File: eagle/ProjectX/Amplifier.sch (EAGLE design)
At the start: 5 parts, among them U1 TC4427COA

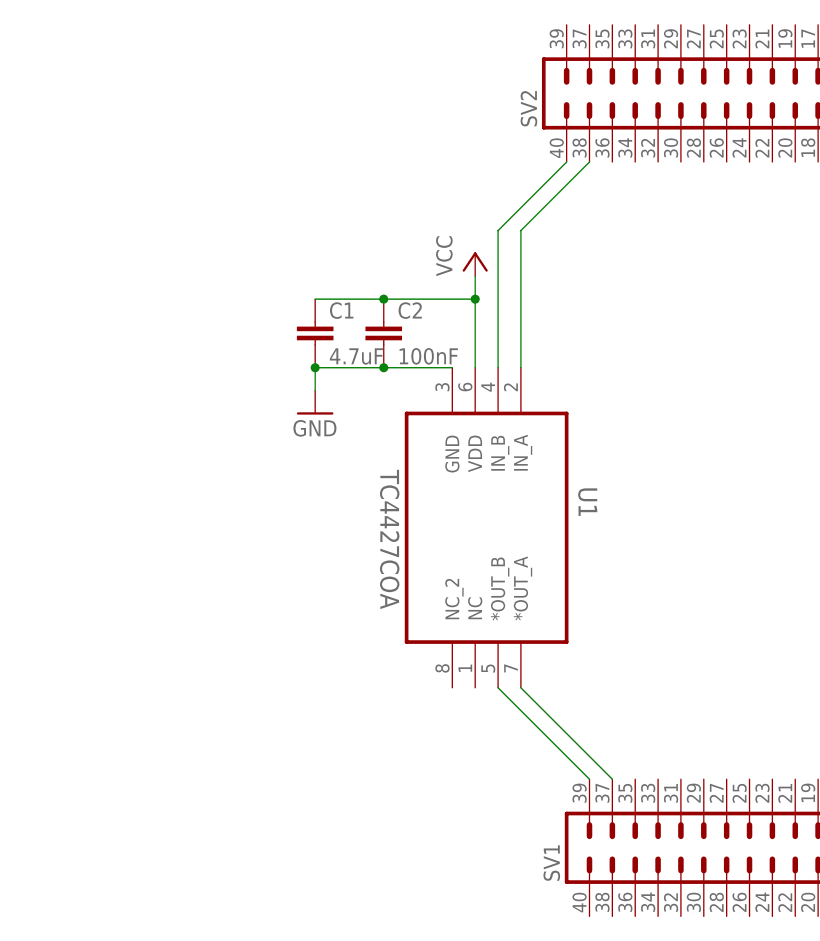
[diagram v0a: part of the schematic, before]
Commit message: Board update
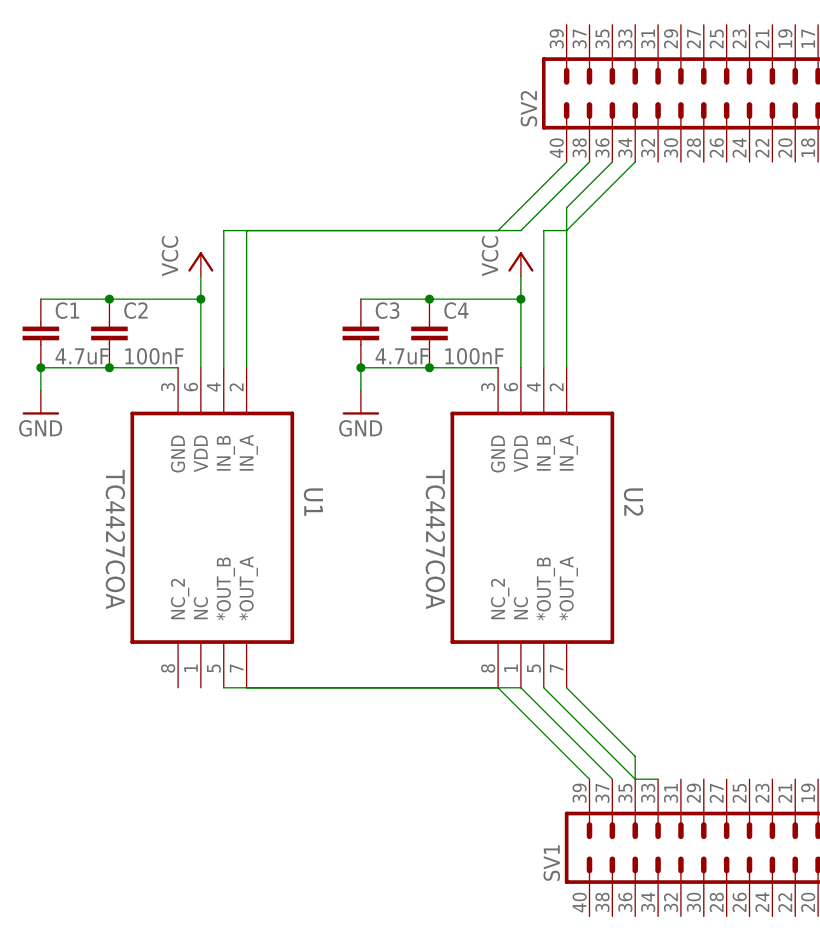
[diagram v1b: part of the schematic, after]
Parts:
- added C3: 4.7uF, rcl:C-EUC0805
- added C4: 100nF, rcl:C-EUC0805
- added U2: TC4427COA, Microchip_By_element14_Batch_1:TC4427COA
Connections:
- new net N$1: SV2.34, U2.IN_B
- new net N$6: SV2.36, U2.IN_A
- new net N$7: SV1.35, U2.*OUT_A
- new net N$8: SV1.33, U2.*OUT_B
- net GND: now also C3.2, C4.2, U2.GND
- net N$2: now also U1.*OUT_A; no longer U1.*OUT_B
- net N$3: now also U1.*OUT_B; no longer U1.*OUT_A
- net N$4: now also SV2.38; no longer SV2.40
- net N$5: now also SV2.40; no longer SV2.38
- net VCC: now also C3.1, C4.1, U2.VDD
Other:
- moved on the sheet: C1, C2, U1
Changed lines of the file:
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@@
 <part name="P+4" library="supply1" library_urn="urn:adsk.eagle:library:371" deviceset="VCC" device=""/>
 <part name="P+5" library="supply1" library_urn="urn:adsk.eagle:library:371" deviceset="VCC" device=""/>
+<part name="U2" library="Microchip_By_element14_Batch_1" deviceset="TC4427COA" device=""/>
+<part name="C3" library="rcl" library_urn="urn:adsk.eagle:library:334" deviceset="C-EU" device="C0805" package3d_urn="urn:adsk.eagle:package:23617/2" value="4.7uF"/>
+<part name="C4" library="rcl" library_urn="urn:adsk.eagle:library:334" deviceset="C-EU" device="C0805" package3d_urn="urn:adsk.eagle:package:23617/2" value="100nF"/>
+<part name="P+6" library="supply1" library_urn="urn:adsk.eagle:library:371" deviceset="VCC" device=""/>
+<part name="GND6" library="supply1" library_urn="urn:adsk.eagle:library:371" deviceset="GND" device=""/>
 </parts>
 <sheets>
@@
 </plain>
 <instances>
-<instance part="U1" gate="A" x="5.08" y="43.18" rot="R270"/>
-<instance part="C1" gate="G$1" x="-17.78" y="66.04"/>
-<instance part="C2" gate="G$1" x="-10.16" y="66.04"/>
+<instance part="U1" gate="A" x="-25.4" y="43.18" rot="R270"/>
+<instance part="C1" gate="G$1" x="-48.26" y="66.04"/>
+<instance part="C2" gate="G$1" x="-40.64" y="66.04"/>
 <instance part="SV1" gate="1" x="35.56" y="7.62" rot="R90"/>
 <instance part="SV2" gate="1" x="33.02" y="91.44" rot="R90"/>
@@
 <instance part="P+1" gate="VCC" x="58.42" y="22.86"/>
 <instance part="P+2" gate="VCC" x="58.42" y="-5.08" rot="R180"/>
-<instance part="P+3" gate="VCC" x="0" y="73.66"/>
-<instance part="GND3" gate="1" x="-17.78" y="55.88"/>
+<instance part="P+3" gate="VCC" x="-30.48" y="73.66"/>
+<instance part="GND3" gate="1" x="-48.26" y="55.88"/>
 <instance part="GND4" gate="1" x="58.42" y="104.14" rot="R180"/>
 <instance part="GND5" gate="1" x="58.42" y="76.2"/>
 <instance part="P+4" gate="VCC" x="55.88" y="78.74" rot="R180"/>
 <instance part="P+5" gate="VCC" x="55.88" y="111.76"/>
+<instance part="U2" gate="A" x="10.16" y="43.18" rot="R270"/>
+<instance part="C3" gate="G$1" x="-12.7" y="66.04"/>
+<instance part="C4" gate="G$1" x="-5.08" y="66.04"/>
+<instance part="P+6" gate="VCC" x="5.08" y="73.66"/>
+<instance part="GND6" gate="1" x="-12.7" y="55.88"/>
 </instances>
 <busses>
@@
 <pinref part="U1" gate="A" pin="VDD"/>
 <pinref part="P+3" gate="VCC" pin="VCC"/>
-<wire x1="0" y1="60.96" x2="0" y2="68.58" width="0.1524" layer="91"/>
+<wire x1="-30.48" y1="60.96" x2="-30.48" y2="68.58" width="0.1524" layer="91"/>
 <pinref part="C2" gate="G$1" pin="1"/>
-<wire x1="0" y1="68.58" x2="0" y2="71.12" width="0.1524" layer="91"/>
-<wire x1="0" y1="68.58" x2="-10.16" y2="68.58" width="0.1524" layer="91"/>
-<junction x="0" y="68.58"/>
+<wire x1="-30.48" y1="68.58" x2="-30.48" y2="71.12" width="0.1524" layer="91"/>
+<wire x1="-30.48" y1="68.58" x2="-40.64" y2="68.58" width="0.1524" layer="91"/>
+<junction x="-30.48" y="68.58"/>
 <pinref part="C1" gate="G$1" pin="1"/>
-<wire x1="-10.16" y1="68.58" x2="-17.78" y2="68.58" width="0.1524" layer="91"/>
-<junction x="-10.16" y="68.58"/>
+<wire x1="-40.64" y1="68.58" x2="-48.26" y2="68.58" width="0.1524" layer="91"/>
+<junction x="-40.64" y="68.58"/>
 </segment>
 <segment>
@@
 <pinref part="P+4" gate="VCC" pin="VCC"/>
 <wire x1="55.88" y1="83.82" x2="55.88" y2="81.28" width="0.1524" layer="91"/>
+</segment>
+<segment>
+<pinref part="U2" gate="A" pin="VDD"/>
+<pinref part="P+6" gate="VCC" pin="VCC"/>
+<wire x1="5.08" y1="60.96" x2="5.08" y2="68.58" width="0.1524" layer="91"/>
+<pinref part="C4" gate="G$1" pin="1"/>
+<wire x1="5.08" y1="68.58" x2="5.08" y2="71.12" width="0.1524" layer="91"/>
+<wire x1="5.08" y1="68.58" x2="-5.08" y2="68.58" width="0.1524" layer="91"/>
+<junction x="5.08" y="68.58"/>
+<pinref part="C3" gate="G$1" pin="1"/>
+<wire x1="-5.08" y1="68.58" x2="-12.7" y2="68.58" width="0.1524" layer="91"/>
+<junction x="-5.08" y="68.58"/>
 </segment>
 </net>
@@
 <pinref part="U1" gate="A" pin="GND"/>
 <pinref part="C2" gate="G$1" pin="2"/>
-<wire x1="-2.54" y1="60.96" x2="-10.16" y2="60.96" width="0.1524" layer="91"/>
+<wire x1="-33.02" y1="60.96" x2="-40.64" y2="60.96" width="0.1524" layer="91"/>
 <pinref part="C1" gate="G$1" pin="2"/>
-<wire x1="-10.16" y1="60.96" x2="-17.78" y2="60.96" width="0.1524" layer="91"/>
-<junction x="-10.16" y="60.96"/>
+<wire x1="-40.64" y1="60.96" x2="-48.26" y2="60.96" width="0.1524" layer="91"/>
+<junction x="-40.64" y="60.96"/>
 <pinref part="GND3" gate="1" pin="GND"/>
-<wire x1="-17.78" y1="58.42" x2="-17.78" y2="60.96" width="0.1524" layer="91"/>
-<junction x="-17.78" y="60.96"/>
+<wire x1="-48.26" y1="58.42" x2="-48.26" y2="60.96" width="0.1524" layer="91"/>
+<junction x="-48.26" y="60.96"/>
 </segment>
 <segment>
@@
 <wire x1="58.42" y1="83.82" x2="58.42" y2="78.74" width="0.1524" layer="91"/>
 </segment>
+<segment>
+<pinref part="U2" gate="A" pin="GND"/>
+<pinref part="C4" gate="G$1" pin="2"/>
+<wire x1="2.54" y1="60.96" x2="-5.08" y2="60.96" width="0.1524" layer="91"/>
+<pinref part="C3" gate="G$1" pin="2"/>
+<wire x1="-5.08" y1="60.96" x2="-12.7" y2="60.96" width="0.1524" layer="91"/>
+<junction x="-5.08" y="60.96"/>
+<pinref part="GND6" gate="1" pin="GND"/>
+<wire x1="-12.7" y1="58.42" x2="-12.7" y2="60.96" width="0.1524" layer="91"/>
+<junction x="-12.7" y="60.96"/>
+</segment>
 </net>
 <net name="N$4" class="0">
 <segment>
-<pinref part="SV2" gate="1" pin="40"/>
-<wire x1="10.16" y1="83.82" x2="2.54" y2="76.2" width="0.1524" layer="91"/>
-<wire x1="2.54" y1="76.2" x2="2.54" y2="60.96" width="0.1524" layer="91"/>
+<wire x1="-27.94" y1="76.2" x2="-27.94" y2="60.96" width="0.1524" layer="91"/>
 <pinref part="U1" gate="A" pin="IN_B"/>
+<pinref part="SV2" gate="1" pin="38"/>
+<wire x1="-27.94" y1="76.2" x2="5.08" y2="76.2" width="0.1524" layer="91"/>
+<wire x1="5.08" y1="76.2" x2="12.7" y2="83.82" width="0.1524" layer="91"/>
 </segment>
 </net>
 <net name="N$5" class="0">
 <segment>
-<pinref part="SV2" gate="1" pin="38"/>
-<wire x1="12.7" y1="83.82" x2="5.08" y2="76.2" width="0.1524" layer="91"/>
-<wire x1="5.08" y1="76.2" x2="5.08" y2="60.96" width="0.1524" layer="91"/>
+<wire x1="-25.4" y1="76.2" x2="-25.4" y2="60.96" width="0.1524" layer="91"/>
 <pinref part="U1" gate="A" pin="IN_A"/>
+<pinref part="SV2" gate="1" pin="40"/>
+<wire x1="-25.4" y1="76.2" x2="2.54" y2="76.2" width="0.1524" layer="91"/>
+<wire x1="2.54" y1="76.2" x2="10.16" y2="83.82" width="0.1524" layer="91"/>
+</segment>
+</net>
+<net name="N$1" class="0">
+<segment>
+<wire x1="7.62" y1="76.2" x2="7.62" y2="60.96" width="0.1524" layer="91"/>
+<pinref part="U2" gate="A" pin="IN_B"/>
+<pinref part="SV2" gate="1" pin="34"/>
+<wire x1="7.62" y1="76.2" x2="10.16" y2="76.2" width="0.1524" layer="91"/>
+<wire x1="10.16" y1="76.2" x2="17.78" y2="83.82" width="0.1524" layer="91"/>
+</segment>
+</net>
+<net name="N$7" class="0">
+<segment>
+<pinref part="SV1" gate="1" pin="35"/>
+<pinref part="U2" gate="A" pin="*OUT_A"/>
+<wire x1="17.78" y1="15.24" x2="17.78" y2="17.78" width="0.1524" layer="91"/>
+<wire x1="17.78" y1="17.78" x2="10.16" y2="25.4" width="0.1524" layer="91"/>
+</segment>
+</net>
+<net name="N$8" class="0">
+<segment>
+<pinref part="SV1" gate="1" pin="33"/>
+<pinref part="U2" gate="A" pin="*OUT_B"/>
+<wire x1="20.32" y1="15.24" x2="17.78" y2="15.24" width="0.1524" layer="91"/>
+<wire x1="17.78" y1="15.24" x2="7.62" y2="25.4" width="0.1524" layer="91"/>
+</segment>
+</net>
+<net name="N$6" class="0">
+<segment>
+<pinref part="U2" gate="A" pin="IN_A"/>
+<pinref part="SV2" gate="1" pin="36"/>
+<wire x1="10.16" y1="60.96" x2="10.16" y2="78.74" width="0.1524" layer="91"/>
+<wire x1="10.16" y1="78.74" x2="15.24" y2="83.82" width="0.1524" layer="91"/>
 </segment>
 </net>
 <net name="N$2" class="0">
 <segment>
-<pinref part="U1" gate="A" pin="*OUT_B"/>
+<pinref part="U1" gate="A" pin="*OUT_A"/>
 <pinref part="SV1" gate="1" pin="39"/>
+<wire x1="-25.4" y1="25.4" x2="2.54" y2="25.4" width="0.1524" layer="91"/>
 <wire x1="2.54" y1="25.4" x2="12.7" y2="15.24" width="0.1524" layer="91"/>
 </segment>
@@
 <net name="N$3" class="0">
 <segment>
-<pinref part="U1" gate="A" pin="*OUT_A"/>
+<pinref part="U1" gate="A" pin="*OUT_B"/>
 <pinref part="SV1" gate="1" pin="37"/>
+<wire x1="-27.94" y1="25.4" x2="5.08" y2="25.4" width="0.1524" layer="91"/>
 <wire x1="5.08" y1="25.4" x2="15.24" y2="15.24" width="0.1524" layer="91"/>
 </segment>

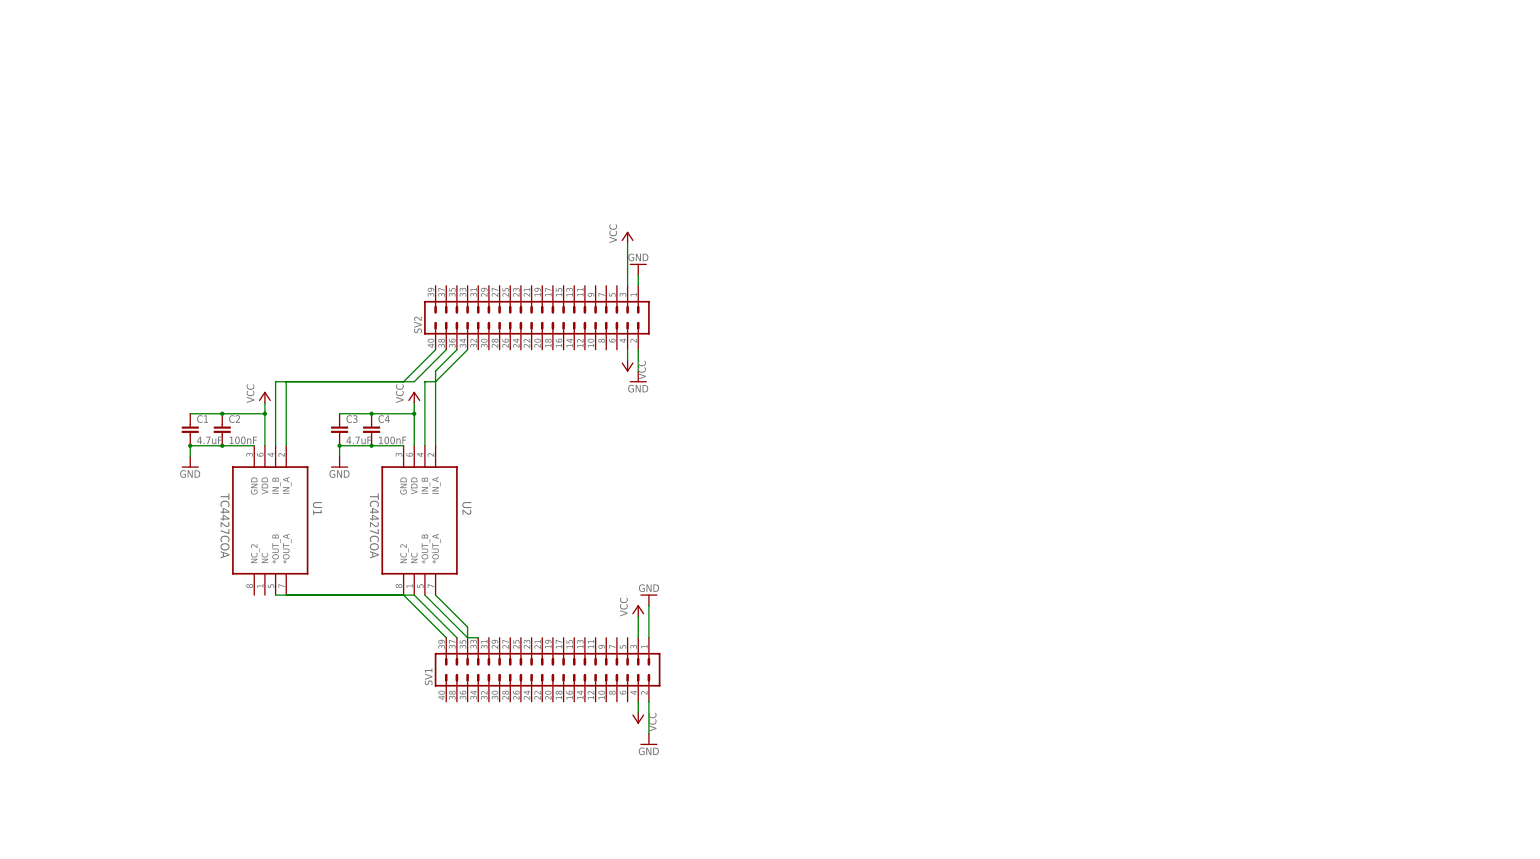
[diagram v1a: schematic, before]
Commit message: changes
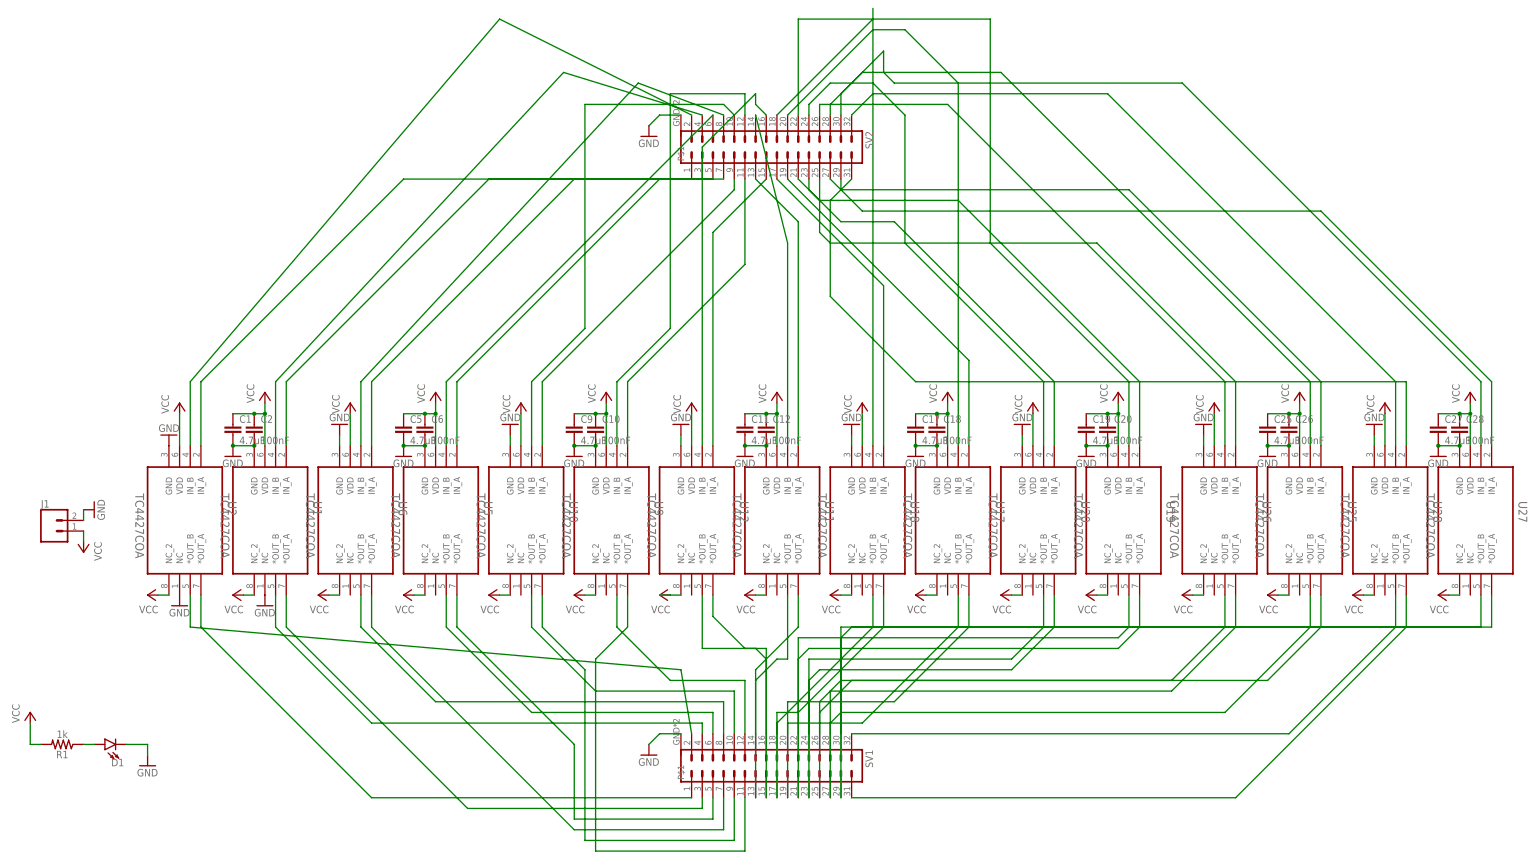
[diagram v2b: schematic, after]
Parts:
- removed C3: 4.7uF, rcl:C-EUC0805
- removed C4: 100nF, rcl:C-EUC0805
- added C10, C12, C18, C20, C26, C28, C6: 100nF, rcl:C-EUC0805
- added C11, C17, C19, C25, C27, C5, C9: 4.7uF, rcl:C-EUC0805
- added D1: (no value), SparkFun-LED:LED0603
- added J1: (no value), SparkFun-Connectors:CONN_02PTH3
- added R1: 1k, SparkFun-Resistors:0.22OHM-0805-1/4W-1%
- added U10, U11, U12, U17, U18, U19, U20, U25, U26, U27, U28, U5, U6, U9: TC4427COA, Microchip_By_element14_Batch_1:TC4427COA
- SV1, SV2: device con-lstb:MA20-2W -> Parts:MA20-2W
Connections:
- removed net VCC: C1.1, C2.1, C3.1, C4.1, SV1.3, SV1.4, SV2.3, SV2.4, U1.VDD, U2.VDD
- new net N$10: SV1.1, U2.*OUT_A
- new net N$100: SV1.25, U26.*OUT_A
- new net N$101: SV1.26, U26.*OUT_B
- new net N$102: SV2.25, U26.IN_A
- new net N$103: SV1.27, U25.*OUT_A
- new net N$104: SV1.28, U25.*OUT_B
- new net N$105: SV2.30, U27.IN_B
- new net N$106: SV2.29, U27.IN_A
- new net N$107: SV2.32, U28.IN_B
- new net N$108: SV1.31, U28.*OUT_A
- new net N$109: SV1.32, U28.*OUT_B
- new net N$11: SV1.3, U1.*OUT_A
- new net N$110: SV2.31, U28.IN_A
- new net N$111: SV1.29, U27.*OUT_A
- new net N$112: SV1.30, U27.*OUT_B
- new net N$12: SV1.7, U6.*OUT_A
- new net N$13: SV1.10, U10.*OUT_B
- new net N$14: SV1.9, U10.*OUT_A
- new net N$15: SV1.11, U9.*OUT_A
- new net N$16: SV1.23, U20.*OUT_A
- new net N$17: SV2.6, U5.IN_B
- new net N$18: SV2.5, U5.IN_A
- new net N$19: SV2.8, U6.IN_B
- new net N$20: D1.A, R1.1
- new net N$22: SV2.7, U6.IN_A
- new net N$23: SV1.5, U5.*OUT_A
- new net N$24: SV1.6, U5.*OUT_B
- new net N$26: SV1.15, U12.*OUT_A
- new net N$29: SV1.12, U9.*OUT_B
- new net N$33: SV2.12, U9.IN_B
- new net N$34: SV2.11, U9.IN_A
- new net N$35: SV2.10, U10.IN_B
- new net N$38: SV2.9, U10.IN_A
- new net N$41: SV2.14, U11.IN_B
- new net N$42: SV2.13, U11.IN_A
- new net N$43: SV2.16, U12.IN_B
- new net N$46: SV2.15, U12.IN_A
- new net N$47: SV1.13, U11.*OUT_A
- new net N$48: SV1.14, U11.*OUT_B
- new net N$65: SV2.20, U17.IN_B
- new net N$66: SV2.19, U17.IN_A
- new net N$67: SV2.18, U18.IN_B
- new net N$68: SV1.17, U18.*OUT_A
- new net N$69: SV1.18, U18.*OUT_B
- new net N$70: SV2.17, U18.IN_A
- new net N$71: SV1.19, U17.*OUT_A
- new net N$72: SV1.20, U17.*OUT_B
- new net N$73: SV2.22, U19.IN_B
- new net N$74: SV2.21, U19.IN_A
- new net N$75: SV2.24, U20.IN_B
- new net N$78: SV2.23, U20.IN_A
- new net N$79: SV1.21, U19.*OUT_A
- new net N$80: SV1.22, U19.*OUT_B
- new net N$9: SV1.8, U6.*OUT_B
- new net N$97: SV2.28, U25.IN_B
- new net N$98: SV2.27, U25.IN_A
- new net N$99: SV2.26, U26.IN_B
- new net VDD: C1.1, C10.1, C11.1, C12.1, C17.1, C18.1, C19.1, C2.1, C20.1, C25.1, C26.1, C27.1, C28.1, C5.1, C6.1, C9.1, J1.1, R1.2, U1.NC_2, U1.VDD, U10.NC_2, U10.VDD, U11.NC_2, U11.VDD, U12.NC_2, U12.VDD, U17.NC_2, U17.VDD, U18.NC_2, U18.VDD, U19.NC_2, U19.VDD, U2.NC_2, U2.VDD, U20.NC_2, U20.VDD, U25.NC_2, U25.VDD, U26.NC_2, U26.VDD, U27.NC_2, U27.VDD, U28.NC_2, U28.VDD, U5.NC_2, U5.VDD, U6.NC_2, U6.VDD, U9.NC_2, U9.VDD
- net GND: now also C10.2, C11.2, C12.2, C17.2, C18.2, C19.2, C20.2, C25.2, C26.2, C27.2, C28.2, C5.2, C6.2, C9.2, D1.C, J1.2, SV1.P$1, SV2.P$1, U1.NC, U10.GND, U10.NC, U11.GND, U11.NC, U12.GND, U12.NC, U17.GND, U17.NC, U18.GND, U18.NC, U19.GND, U19.NC, U2.NC, U20.GND, U20.NC, U25.GND, U25.NC, U26.GND, U26.NC, U27.GND, U27.NC, U28.GND, U28.NC, U5.GND, U5.NC, U6.GND, U6.NC, U9.GND, U9.NC; no longer C3.2, C4.2, SV1.1, SV1.2, SV2.1, SV2.2
- net N$1: now also SV2.2; no longer SV2.34
- net N$2: now also SV1.2, U2.*OUT_B; no longer SV1.39, U1.*OUT_A
- net N$3: now also SV1.4; no longer SV1.37
- net N$4: now also SV2.4; no longer SV2.38
- net N$5: now also SV2.3; no longer SV2.40
- net N$6: now also SV2.1; no longer SV2.36
- net N$7: now also SV1.16, U12.*OUT_B; no longer SV1.35, U2.*OUT_A
- net N$8: now also SV1.24, U20.*OUT_B; no longer SV1.33, U2.*OUT_B
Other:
- moved on the sheet: C1, C2, U2
